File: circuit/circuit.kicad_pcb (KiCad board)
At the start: 2 copper layers, 52 parts, among them J1 Conn_01x20_Female, J2 Conn_02x03_Odd_Even, P1 CONN_02X03, U1 LMC6484, U10 ATmega328P-PU, U2 LIS3DHTR, U3 LM358DT, U4 LM358DT, U5 L78M05CDT-TR, U6 LM3480, U7 SN74LV4052APWR, U8 SN74LV4052APWR, U9 DRV8834, Y1 Crystal_SMD

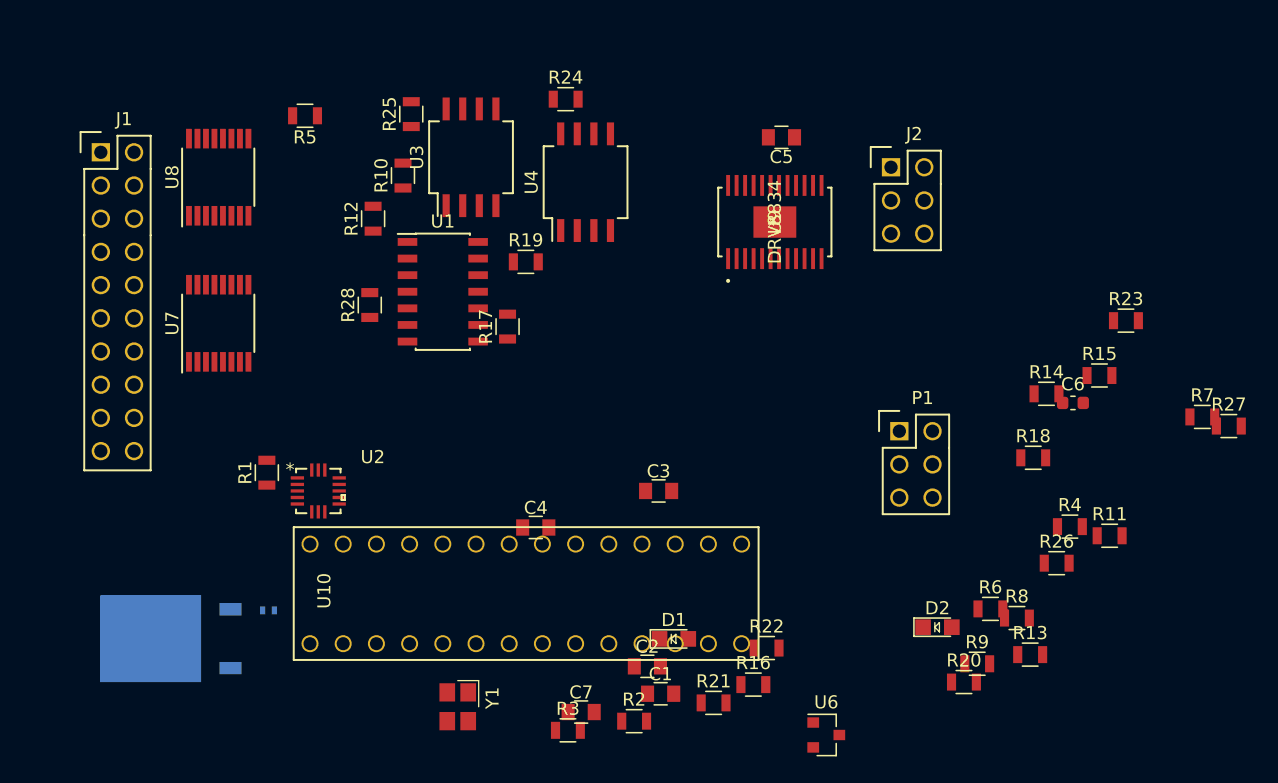
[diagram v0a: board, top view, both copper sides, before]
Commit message: started on layout. *make crab noise*
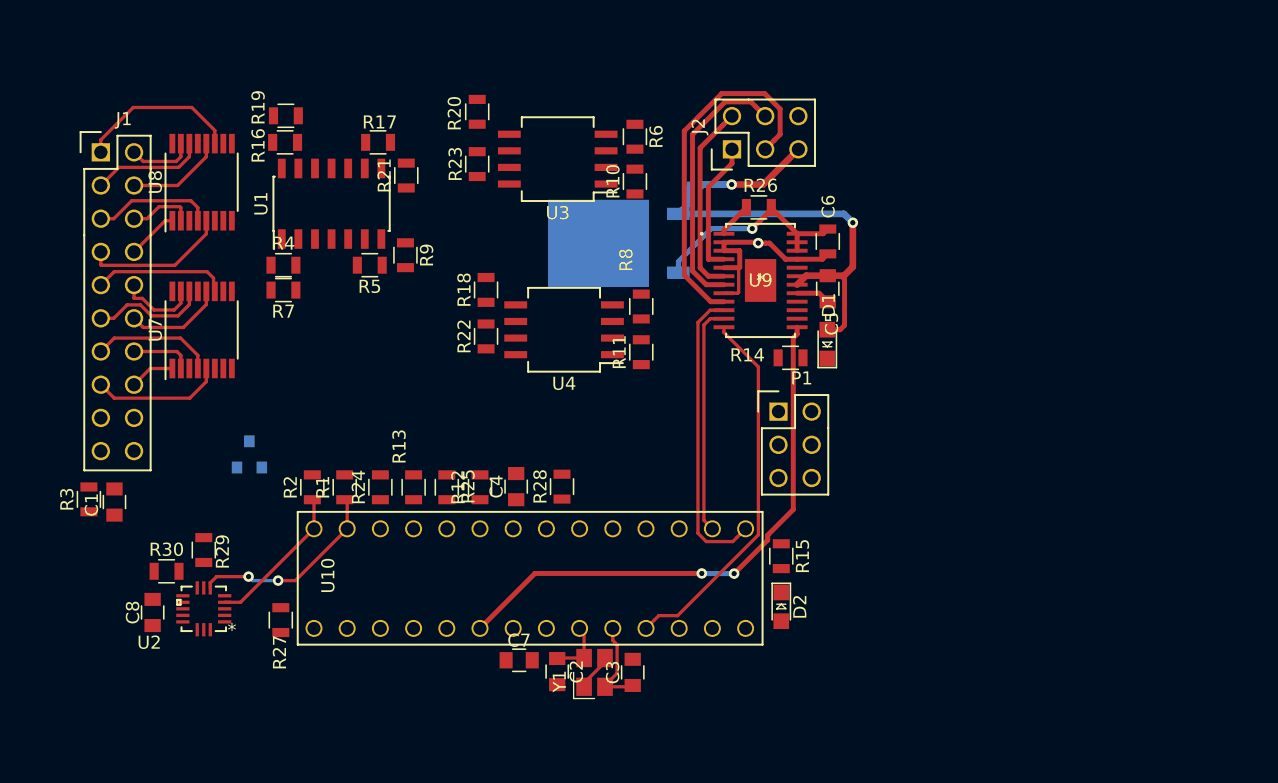
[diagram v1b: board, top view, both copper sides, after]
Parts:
- added C8: C_0.1uF, footprints:C_0805_OEM, F.Cu at (138.2, 99.7)
- added R29: R_10K, footprints:R_0805_OEM, F.Cu at (142.1, 94.9)
- added R30: R_10K, footprints:R_0805_OEM, F.Cu at (139.3, 96.6)
- C6: footprint footprints:C_0603_1608Metric -> footprints:R_0805_OEM
- F1: value Fuse_2A -> Fuse_1A
- U6: moved to B.Cu
- moved R27 74.0 mm to (148.0, 100.3), turned to 270 degrees
- moved R7 71.0 mm to (148.2, 75.1), turned to 180 degrees
- moved R4 63.4 mm to (148.2, 73.2)
- moved R20 57.4 mm to (163.0, 61.4), turned to 270 degrees
- moved R16 54.8 mm to (148.3, 63.8)
- moved R9 53.8 mm to (157.5, 72.4), turned to 270 degrees
- moved R23 51.1 mm to (163.0, 65.4), turned to 90 degrees
- moved U6 49.1 mm to (145.6, 87.6), turned to 90 degrees
- moved R13 48.9 mm to (158.2, 90.1), turned to 90 degrees
- moved R21 46.7 mm to (157.6, 66.3), turned to 90 degrees
- moved F1 46.1 mm to (179.7, 67.1)
- moved U5 45.7 mm to (172.3, 71.5)
- moved R6 45.2 mm to (175.1, 63.3), turned to 270 degrees
- moved C1 44.3 mm to (135.3, 91.3), turned to 90 degrees
- moved R18 43.8 mm to (163.7, 75.0), turned to 270 degrees
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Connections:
- U2 pad 8: VCC -> Net-(R30-Pad2)
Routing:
- net /motorA_DIR: track 0.00 -> 42.0 mm, vias 0 -> 2
- net /battery+: track 0.00 -> 30.7 mm, vias 0 -> 1
- net /motorB_DIR: track 0.00 -> 28.5 mm
- net /motorB+: track 0.00 -> 27.5 mm
- net /motorA_PWM: track 0.00 -> 22.8 mm
- net /motorB-: track 0.00 -> 20.3 mm
- net GND: track 0.00 -> 20.0 mm, vias 0 -> 1
- net /motorB_PWM: track 0.00 -> 17.6 mm
- net VCC: track 0.00 -> 16.4 mm, vias 0 -> 1
- net /SDA: track 0.00 -> 15.1 mm, vias 0 -> 2
- net /motorA-: track 0.00 -> 14.7 mm
- net /red_8: track 0.00 -> 12.4 mm
- net /SCL: track 0.00 -> 11.4 mm
- net /blue_6: track 0.00 -> 11.1 mm
- net /motorA+: track 0.00 -> 10.3 mm
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
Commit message: finished board
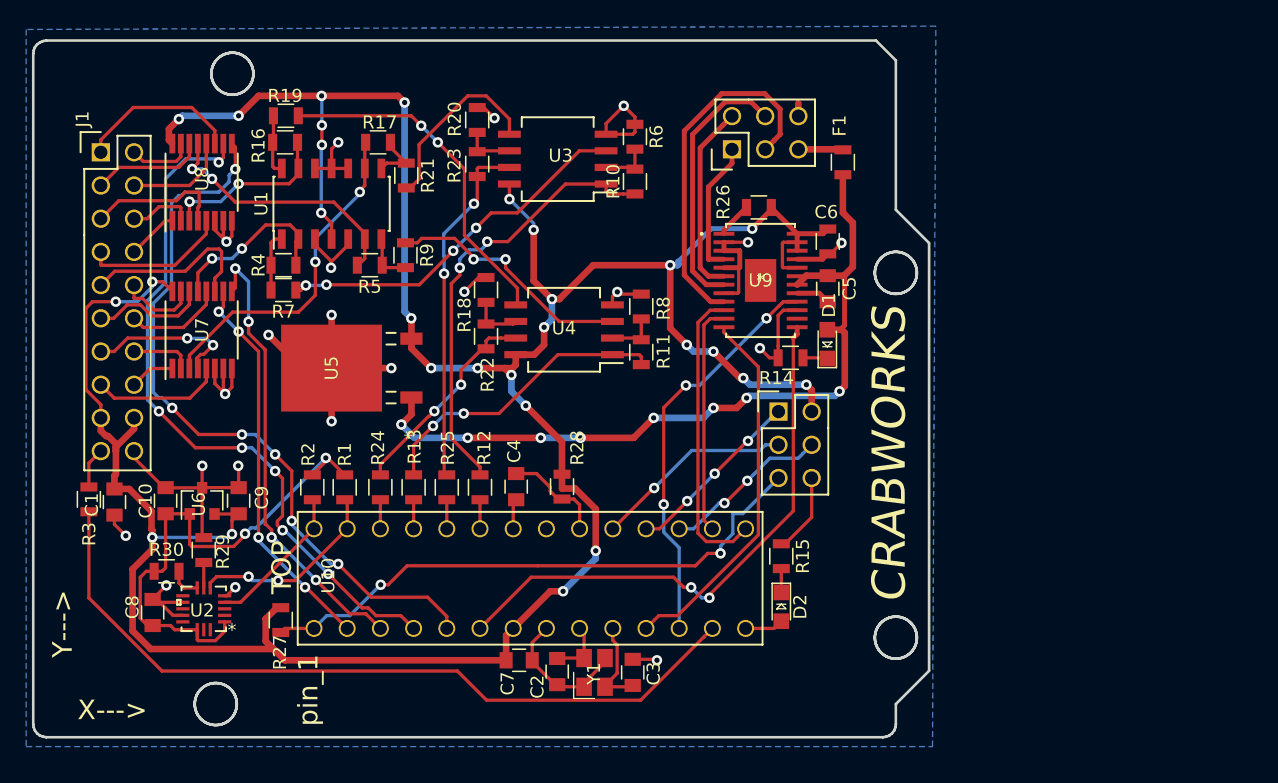
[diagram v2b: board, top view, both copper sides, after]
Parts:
- added C10: C_0.1uF, footprints:C_0805_OEM, F.Cu at (139.2, 91.2)
- added C9: C_0.1uF, footprints:C_0805_OEM, F.Cu at (144.8, 91.2)
- added G***: LOGO, footprints:crab, B.Cu at (162.8, 81.3)
- F1: footprint Resistors_SMD:R_0402 -> footprints:R_0805_OEM; moved to F.Cu
- U5, U6: moved to F.Cu
- moved U5 22.5 mm to (151.9, 81.0), turned to 90 degrees
- moved F1 11.4 mm to (191.0, 65.3), turned to 90 degrees
- moved U6 5.07 mm to (142.0, 91.2)
- moved R20 0.62 mm to (163.0, 62.0)
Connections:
- F1 pad 1: Net-(F1-Pad1) -> /battery+
- F1 pad 2: /battery+ -> Net-(F1-Pad2)
- J2 pad 5: Net-(F1-Pad1) -> Net-(F1-Pad2)
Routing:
- net VCC: track 16.4 -> 241.5 mm, vias 1 -> 28
- net GND: track 20.0 -> 124.5 mm, vias 1 -> 21
- net /led_D1: track 0.00 -> 59.8 mm
- net /select_1B: track 0.00 -> 56.3 mm, vias 0 -> 6
- net /select_0B: track 0.00 -> 54.1 mm, vias 0 -> 6
- net /RESET: track 0.00 -> 44.2 mm, vias 0 -> 2
- net /3.3V: track 0.00 -> 39.4 mm, vias 0 -> 2
- net /select_1A: track 0.00 -> 34.8 mm, vias 0 -> 4
- net Net-(R10-Pad1): track 0.00 -> 34.2 mm, vias 0 -> 2
- net /issues: track 0.00 -> 31.8 mm, vias 0 -> 3
- net /battery+: track 30.7 -> 62.5 mm, vias 1 -> 8
- net /select_0A: track 0.00 -> 30.0 mm, vias 0 -> 4
- net Net-(R7-Pad1): track 0.00 -> 28.1 mm, vias 0 -> 4
- net Net-(R23-Pad1): track 0.00 -> 27.1 mm, vias 0 -> 2
- net Net-(R19-Pad1): track 0.00 -> 26.5 mm, vias 0 -> 2
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- added copper zone on B.Cu, net GND
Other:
- board outline added: 68.5 x 53.3 mm
- board text added: "CRABWORKS"
- board text added: "TOP"
- board text added: "Will Fairman REV_1 -- 11/6/17"
- board text added: "X--->"
- board text added: "Y--->"
- board text added: "pin_1"
